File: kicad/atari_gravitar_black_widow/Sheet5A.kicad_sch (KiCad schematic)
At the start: 121 parts, among them Q2 2N6044, Q3 2N6044, Q4 2N6044

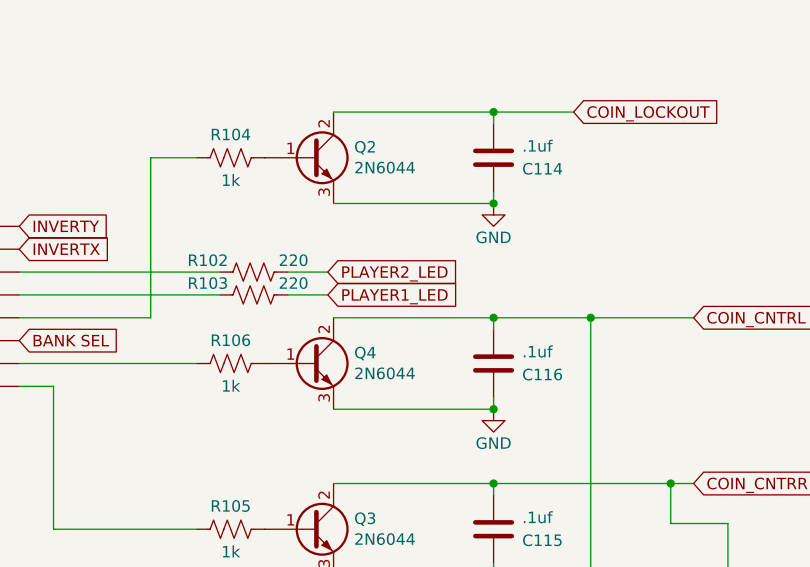
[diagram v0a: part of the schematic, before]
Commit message: push
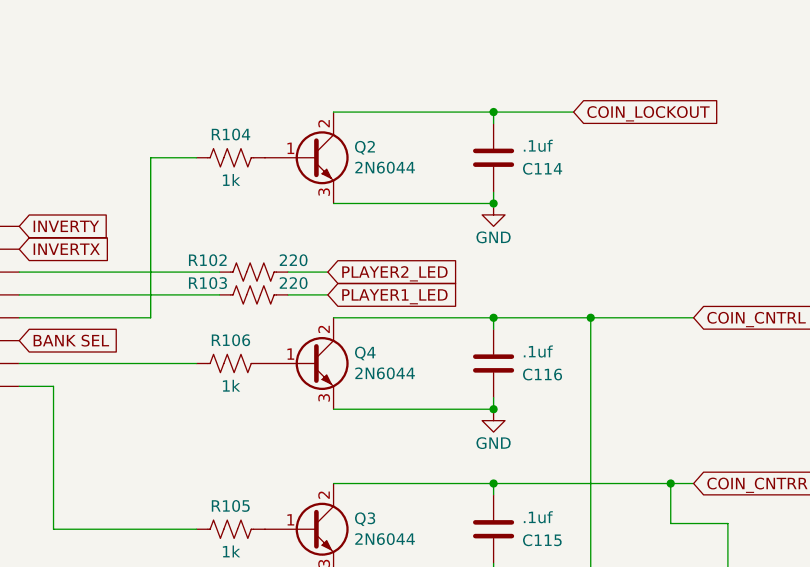
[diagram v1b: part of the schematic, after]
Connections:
- net PLAYER1_LED: now also R103.1
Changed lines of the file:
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@@
     )
   )
-  (global_label "PLAYER1_LED" (shape input) (at 358.78 283.21 0) (fields_autoplaced)
-    (effects (font (size 1.27 1.27)) (justify left))
-    (property "Intersheet References" "${INTERSHEET_REFS}" (id 0) (at 373.6228 283.1306 0)
+  (global_label "PLAYER1_LED" (shape input) (at 358.775 283.21 0) (fields_autoplaced)
+    (effects (font (size 1.27 1.27)) (justify left))
+    (property "Intersheet References" "${INTERSHEET_REFS}" (id 0) (at 373.6178 283.1306 0)
       (effects (font (size 1.27 1.27)) (justify left) hide)
     )
@@
     )
   )
-  (global_label "PLAYER2_LED" (shape input) (at 358.77 280.67 0) (fields_autoplaced)
-    (effects (font (size 1.27 1.27)) (justify left))
-    (property "Intersheet References" "${INTERSHEET_REFS}" (id 0) (at 373.6128 280.5906 0)
-      (effects (font (size 1.27 1.27)) (justify left) hide)
-    )
+  (global_label "PLAYER2_LED" (shape input) (at 358.775 280.67 0) (fields_autoplaced)
+    (effects (font (size 1.27 1.27)) (justify left))
+    (property "Intersheet References" "${INTERSHEET_REFS}" (id 0) (at 373.6178 280.5906 0)
+      (effects (font (size 1.27 1.27)) (justify left) hide)
+    )
